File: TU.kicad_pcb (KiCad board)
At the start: 4 copper layers, 50.8 x 109.2 mm, 134 parts, among them J1 Conn_01x06_Male, J2 Conn_01x17_Male, J3 Conn_01x05_Male, J4 Debugger connector, J5 ARM_JTAG_SWD_10, J6 Conn_01x05_Male, J7 RF_Shield_One_Piece, U1 ADP150AUJZ-3.3-R7, U2 SN65HVD233, U3 CC1200, U4 STM32F407VGTx, U5 CC1190, U6 SN65HVD233, Y1 Crystal_GND24

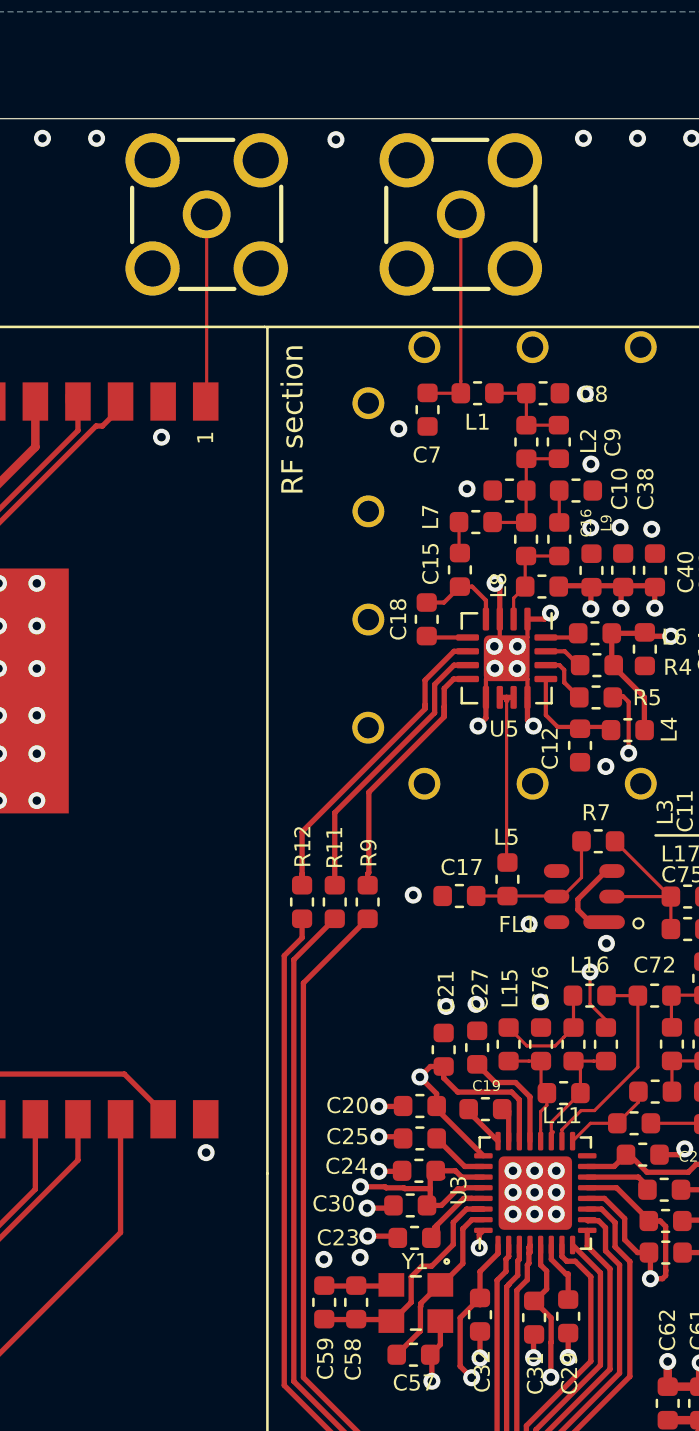
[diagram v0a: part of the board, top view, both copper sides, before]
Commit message: Small changes to routing
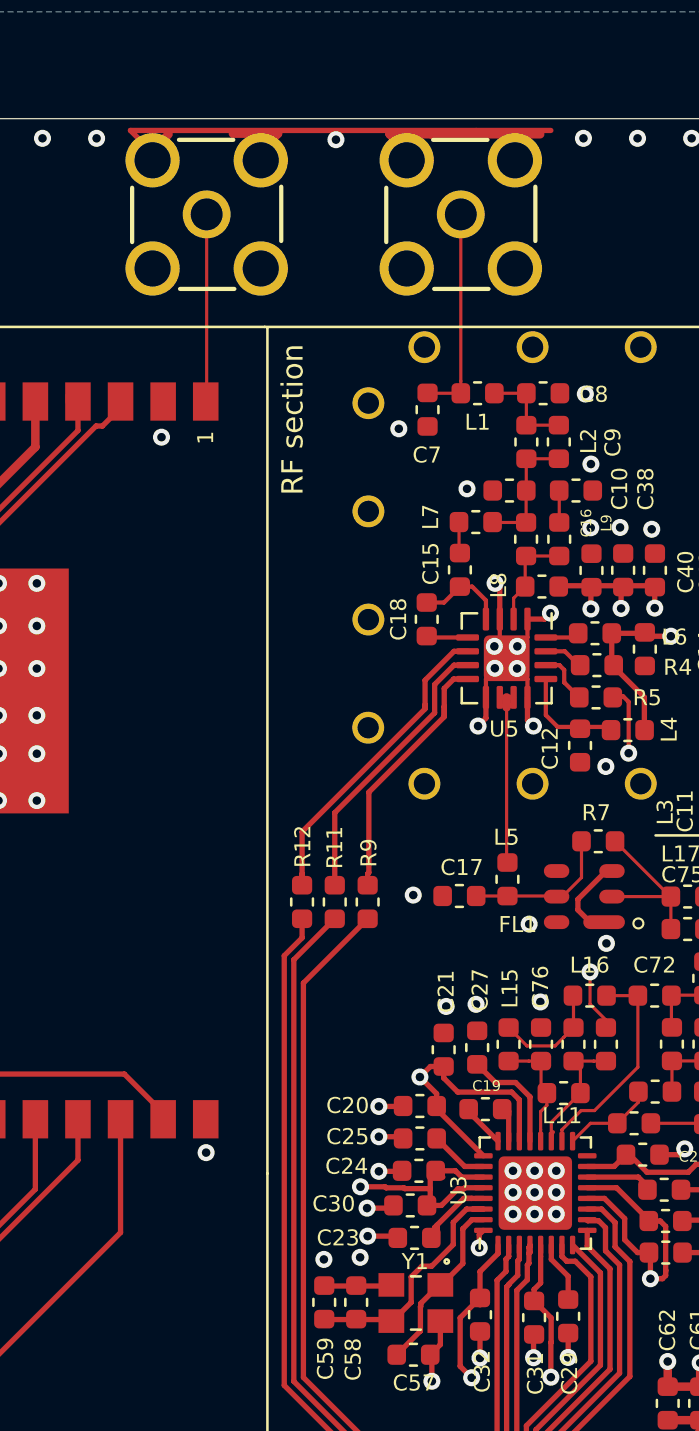
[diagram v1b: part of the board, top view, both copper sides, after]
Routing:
- net GND: track 92.4 -> 128.2 mm
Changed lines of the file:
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@@
     (thickness 1.6)
     (drawings 67)
-    (tracks 1086)
+    (tracks 1102)
     (zones 0)
     (modules 134)
@@
   (segment (start 98.47742 85.2931) (end 98.52976 85.24076) (width 0.25) (layer F.Cu) (net 1) (status 30))
   (segment (start 95.3262 85.2931) (end 98.47742 85.2931) (width 0.25) (layer F.Cu) (net 1) (status 30))
-  (via (at 100.4316 89.7636) (size 0.8) (drill 0.4) (layers F.Cu B.Cu) (net 1))
   (segment (start 100.4316 88.5951) (end 100.3555 88.519) (width 0.25) (layer F.Cu) (net 1) (status 30))
-  (segment (start 100.4316 89.7636) (end 100.4316 88.5951) (width 0.25) (layer F.Cu) (net 1) (status 20))
   (segment (start 99.0001 78.2828) (end 99.0809 78.3636) (width 0.25) (layer F.Cu) (net 1) (status 30))
   (segment (start 97.9424 78.2828) (end 99.0001 78.2828) (width 0.25) (layer F.Cu) (net 1) (status 20))
@@
   (segment (start 98.75002 82.95132) (end 98.8313 83.0326) (width 0.25) (layer F.Cu) (net 1) (status 30))
   (segment (start 97.41916 82.95132) (end 98.75002 82.95132) (width 0.25) (layer F.Cu) (net 1) (status 20))
-  (via (at 95.36176 84.04352) (size 0.8) (drill 0.4) (layers F.Cu B.Cu) (net 1))
-  (via (at 97.06356 83.947) (size 0.8) (drill 0.4) (layers F.Cu B.Cu) (net 1))
   (via (at 117.6655 128.651) (size 0.8) (drill 0.4) (layers F.Cu B.Cu) (net 1))
   (segment (start 109.67199 57.86333) (end 109.67199 60.27407) (width 0.2) (layer F.Cu) (net 1))
@@
   (segment (start 108.613 65.80774) (end 107.288 67.13274) (width 0.25) (layer F.Cu) (net 1))
   (segment (start 108.888 65.80774) (end 108.613 65.80774) (width 0.25) (layer F.Cu) (net 1))
+  (segment (start 100.4316 89.7636) (end 100.4316 88.5951) (width 0.25) (layer F.Cu) (net 1) (status 20))
+  (via (at 100.4316 89.7636) (size 0.8) (drill 0.4) (layers F.Cu B.Cu) (net 1))
+  (via (at 95.36176 84.04352) (size 0.8) (drill 0.4) (layers F.Cu B.Cu) (net 1))
+  (via (at 97.06356 83.947) (size 0.8) (drill 0.4) (layers F.Cu B.Cu) (net 1))
+  (segment (start 87.31758 32.4358) (end 87.31758 31.99346) (width 0.25) (layer F.Cu) (net 1))
+  (segment (start 86.27868 31.03456) (end 102.50868 31.03456) (width 0.25) (layer F.Cu) (net 1))
+  (segment (start 102.50868 31.03456) (end 106.01868 31.03456) (width 0.25) (layer F.Cu) (net 1))
+  (segment (start 99.2505 32.4358) (end 99.2505 32.01638) (width 0.4) (layer F.Cu) (net 1))
+  (segment (start 99.2505 32.01638) (end 98.44868 31.21456) (width 0.4) (layer F.Cu) (net 1))
+  (segment (start 98.44868 31.21456) (end 100.39868 31.21456) (width 0.4) (layer F.Cu) (net 1))
+  (segment (start 100.39868 31.21456) (end 105.51868 31.21456) (width 0.4) (layer F.Cu) (net 1))
+  (segment (start 92.39758 32.4358) (end 92.39758 31.99566) (width 0.4) (layer F.Cu) (net 1))
+  (segment (start 92.39758 31.99566) (end 93.20868 31.18456) (width 0.4) (layer F.Cu) (net 1))
+  (segment (start 93.20868 31.18456) (end 91.08868 31.18456) (width 0.4) (layer F.Cu) (net 1))
+  (segment (start 87.31758 32.4358) (end 87.31758 31.96566) (width 0.4) (layer F.Cu) (net 1))
+  (segment (start 87.31758 31.96566) (end 88.06868 31.21456) (width 0.4) (layer F.Cu) (net 1))
+  (segment (start 87.31758 32.07346) (end 86.27868 31.03456) (width 0.25) (layer F.Cu) (net 1))
+  (segment (start 87.31758 32.4358) (end 87.31758 32.07346) (width 0.25) (layer F.Cu) (net 1))
   (segment (start 101.45996 132.41162) (end 101.34288 132.29454) (width 0.4) (layer F.Cu) (net 2) (status 30))
   (segment (start 101.45996 134.1335) (end 101.45996 132.41162) (width 0.4) (layer F.Cu) (net 2) (status 30))
@@
   (segment (start 100.6559 79.8876) (end 100.9473 80.179) (width 0.25) (layer F.Cu) (net 16) (status 30))
   (segment (start 105.53876 85.72324) (end 105.3592 85.9028) (width 0.25) (layer F.Cu) (net 16) (status 30))
-  (segment (start 105.820812 85.441188) (end 105.820812 84.586412) (width 0.25) (layer F.Cu) (net 16))
-  (segment (start 105.3592 85.9028) (end 105.820812 85.441188) (width 0.25) (layer F.Cu) (net 16) (status 10))
   (via (at 106.0196 89.5731) (size 0.8) (drill 0.4) (layers F.Cu B.Cu) (net 16))
-  (segment (start 105.53876 84.30436) (end 105.53876 83.3665) (width 0.25) (layer F.Cu) (net 16) (status 20))
-  (segment (start 105.820812 84.586412) (end 105.53876 84.30436) (width 0.25) (layer F.Cu) (net 16))
   (segment (start 102.85126 80.179) (end 101.83489 80.179) (width 0.25) (layer F.Cu) (net 16) (status 10))
   (segment (start 100.3554 80.1371) (end 100.6095 79.883) (width 0.25) (layer F.Cu) (net 16) (status 30))
@@
   (segment (start 114.8462 79.5782) (end 115.2989 79.1255) (width 0.25) (layer F.Cu) (net 16))
   (segment (start 113.411 79.5782) (end 114.8462 79.5782) (width 0.25) (layer F.Cu) (net 16))
+  (segment (start 105.53876 83.904) (end 105.53876 83.3665) (width 0.25) (layer F.Cu) (net 16))
+  (segment (start 105.53876 85.14754) (end 105.53876 83.904) (width 0.25) (layer F.Cu) (net 16))
+  (segment (start 105.2322 85.4541) (end 105.53876 85.14754) (width 0.25) (layer F.Cu) (net 16))
+  (segment (start 105.2322 85.9916) (end 105.2322 85.4541) (width 0.25) (layer F.Cu) (net 16))
   (segment (start 102.31376 81.179) (end 102.85126 81.179) (width 0.25) (layer F.Cu) (net 17) (status 20))
   (segment (start 102.092918 81.179) (end 102.31376 81.179) (width 0.25) (layer F.Cu) (net 17))
@@
   (segment (start 102.56012 74.88438) (end 103.41312 75.73738) (width 0.25) (layer F.Cu) (net 19) (status 10))
   (segment (start 103.41312 75.73738) (end 104.364085 75.737381) (width 0.25) (layer F.Cu) (net 19))
-  (segment (start 106.03876 84.04041) (end 106.03876 83.3665) (width 0.25) (layer F.Cu) (net 20) (status 20))
-  (segment (start 106.726548 84.728198) (end 106.03876 84.04041) (width 0.25) (layer F.Cu) (net 20))
-  (segment (start 106.8324 84.728198) (end 106.726548 84.728198) (width 0.25) (layer F.Cu) (net 20))
-  (segment (start 106.8324 85.9281) (end 106.8324 84.728198) (width 0.25) (layer F.Cu) (net 20) (status 10))
+  (segment (start 106.8324 84.83405) (end 106.8324 85.9281) (width 0.25) (layer F.Cu) (net 20))
+  (segment (start 106.03876 83.3665) (end 106.03876 84.04041) (width 0.25) (layer F.Cu) (net 20))
+  (segment (start 106.03876 84.04041) (end 106.8324 84.83405) (width 0.25) (layer F.Cu) (net 20))
   (segment (start 106.4125 47.94382) (end 106.41118 47.9425) (width 0.15) (layer F.Cu) (net 21))
   (segment (start 106.4125 49.441) (end 106.4125 47.94382) (width 0.15) (layer F.Cu) (net 21))
@@
   (segment (start 94.33814 68.94699) (end 93.49998 69.78515) (width 0.25) (layer F.Cu) (net 42))
   (segment (start 94.33814 68.04924) (end 94.33814 68.94699) (width 0.25) (layer F.Cu) (net 42) (status 10))
-  (segment (start 93.49998 69.78515) (end 93.499981 89.958191) (width 0.25) (layer F.Cu) (net 42))
   (segment (start 93.499981 89.958191) (end 96.456 92.91421) (width 0.25) (layer F.Cu) (net 42))
+  (segment (start 93.49998 69.78515) (end 93.499981 89.958191) (width 0.25) (layer F.Cu) (net 42))
   (segment (start 96.956 92.7778) (end 96.956 99.6654) (width 0.25) (layer F.Cu) (net 43) (status 20))
   (segment (start 96.956 92.7778) (end 93.94999 89.77179) (width 0.25) (layer F.Cu) (net 43))
@@
   (segment (start 103.941039 57.789239) (end 103.95 57.7982) (width 0.25) (layer F.Cu) (net 86))
   (segment (start 103.941039 57.653761) (end 103.941039 57.789239) (width 0.25) (layer F.Cu) (net 86))
-  (segment (start 103.941039 57.789239) (end 103.941039 65.40808) (width 0.15) (layer F.Cu) (net 86))
+  (segment (start 103.941039 57.653761) (end 103.941039 58.032201) (width 0.4) (layer F.Cu) (net 86))
+  (segment (start 103.941039 57.789239) (end 103.941039 58.032201) (width 0.15) (layer F.Cu) (net 86))
+  (segment (start 103.941039 58.032201) (end 103.941039 58.122201) (width 0.4) (layer F.Cu) (net 86))
+  (segment (start 103.941039 58.122201) (end 103.941039 65.40808) (width 0.15) (layer F.Cu) (net 86))
   (segment (start 107.106699 54.841261) (end 107.30288 54.64508) (width 0.2) (layer F.Cu) (net 87) (status 30))
   (segment (start 105.782839 54.841261) (end 107.106699 54.841261) (width 0.2) (layer F.Cu) (net 87) (status 30))
